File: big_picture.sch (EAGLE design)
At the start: 13 parts, among them K1 RELAY-SPDT-JZC-11F, M1 MOTOR10MM

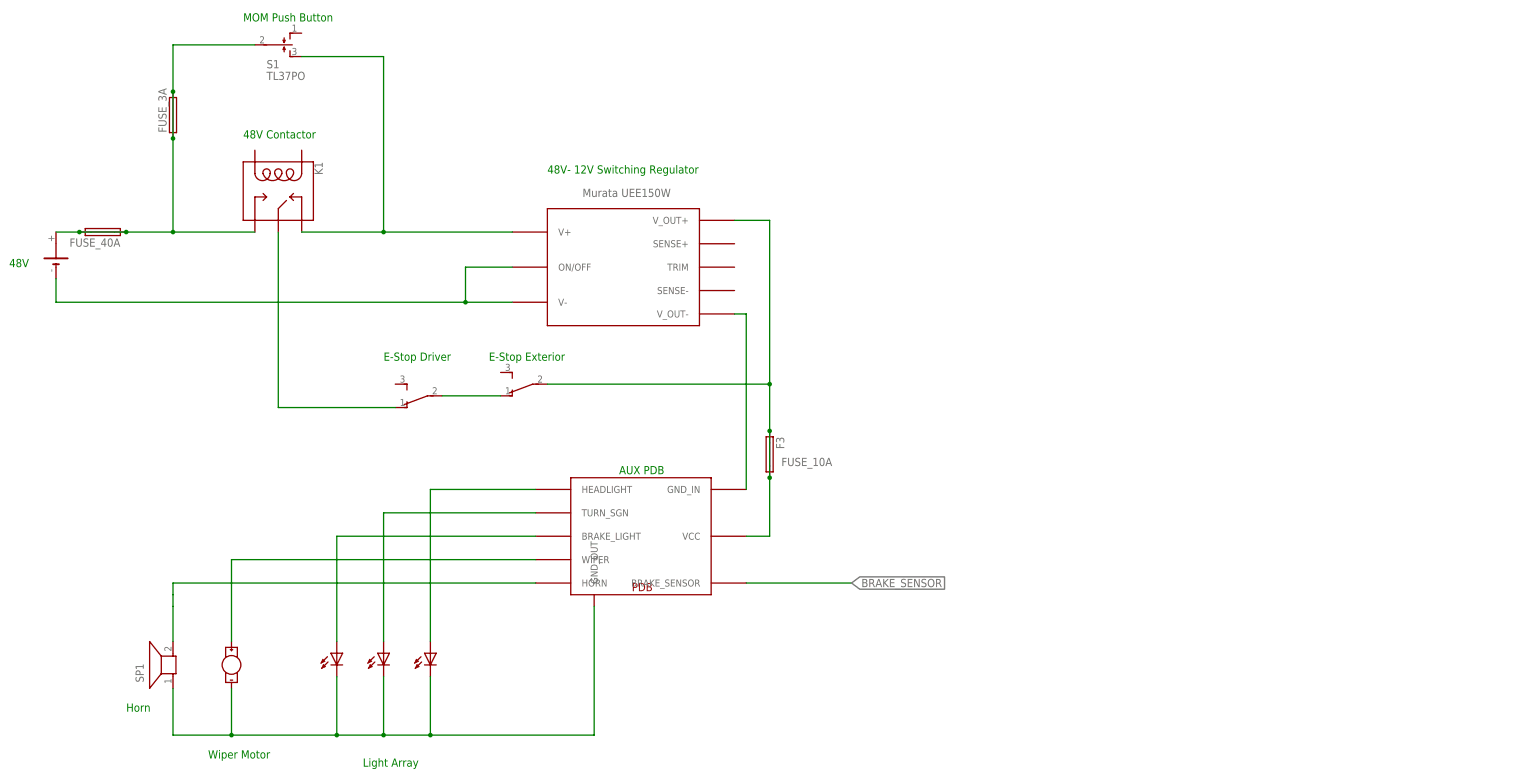
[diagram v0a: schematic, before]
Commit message: Built ESD
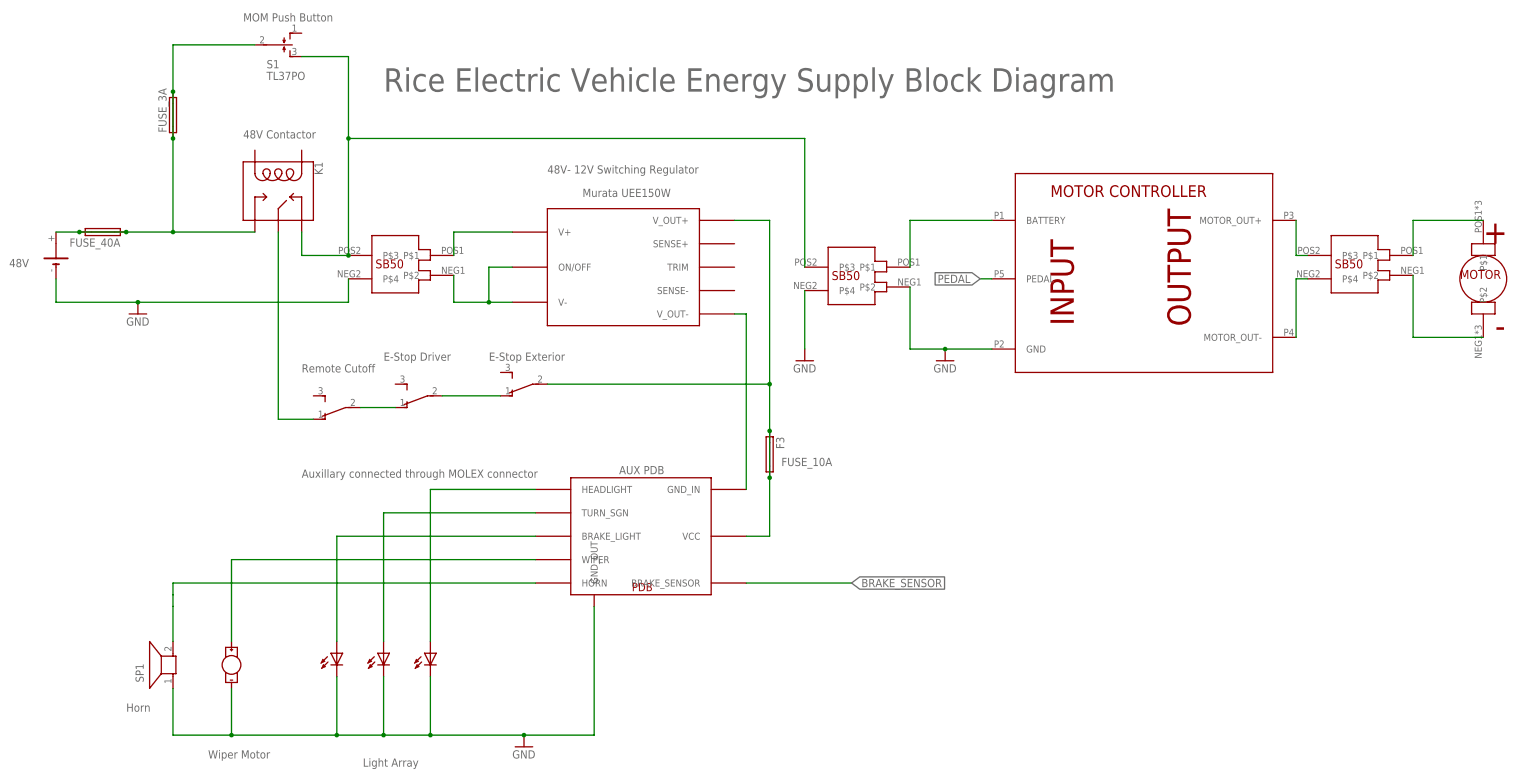
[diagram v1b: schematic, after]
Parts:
- added E_STOP2: TL36WO, switch:TL36WO
- added MOTOR: MOTOR, master_library:MOTOR
- added U$6, U$8, U$9: SB50_BLOCK, master_library:SB50_BLOCK
- added U$7: MOTORCONTROLBLOCK, master_library:MOTORCONTROLBLOCK
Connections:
- removed net N$35: K1.NC, S1.S, U$4.V+
- removed net PDB_GND: DZ1-1.C, DZ1-2.C, DZ1-3.C, M1.-, SP1.1, U$5.GND_OUT
- new net GND: DZ1-1.C, DZ1-2.C, DZ1-3.C, G1.-, M1.-, SP1.1, U$5.GND_OUT, U$6.P$4, U$9.P$4
- new net N$1: U$7.MOTOR_OUT-, U$8.P$4
- new net N$11: E_STOP.O, E_STOP2.P
- new net N$12: U$6.P$1, U$7.BATTERY
- new net N$13: MOTOR.P$1, U$8.P$1
- new net N$14: MOTOR.P$2, U$8.P$2
- new net N$15: U$4.ON/OFF, U$4.V-, U$9.P$2
- new net N$16: K1.NC, S1.S, U$6.P$3, U$9.P$3
- new net N$17: U$4.V+, U$9.P$1
- new net N$6: U$7.MOTOR_OUT+, U$8.P$3
- new net PEDAL: U$7.PEDAL
- net N$4: now also U$6.P$2, U$7.GND; no longer G1.-, U$4.ON/OFF, U$4.V-
- net N$7: now also E_STOP2.O; no longer E_STOP.O
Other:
- note added: "Auxillary connected through MOLEX connector"
- note added: "Remote Cutoff"
- note added: "Rice Electric Vehicle Energy Supply Block Diagram"
